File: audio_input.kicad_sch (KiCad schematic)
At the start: 7 parts

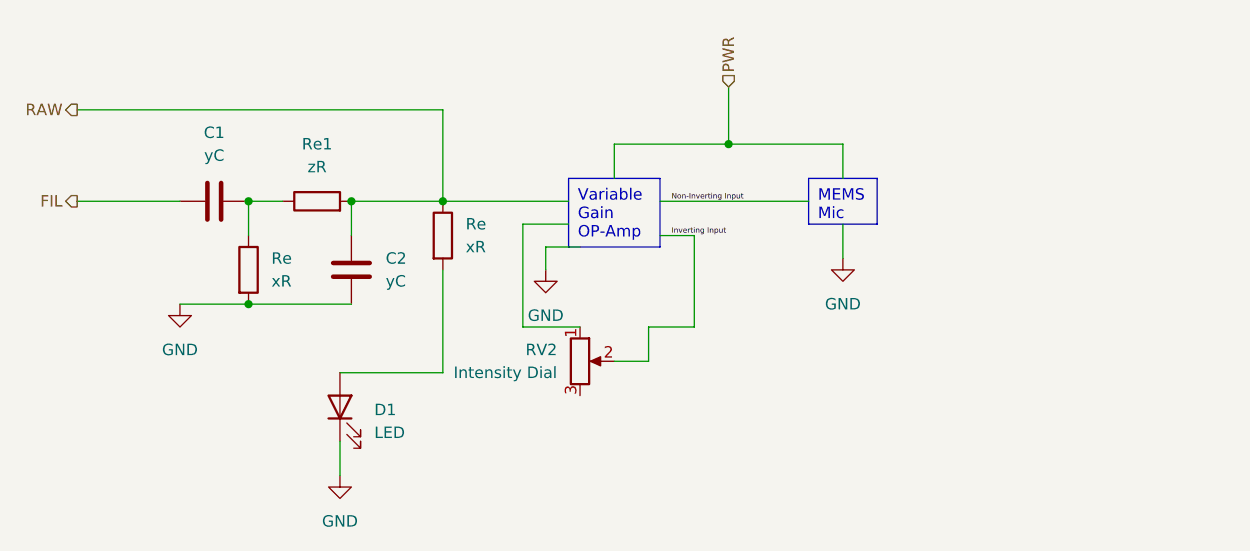
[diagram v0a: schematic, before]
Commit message: started work on pcb layout
started work on pcb layout
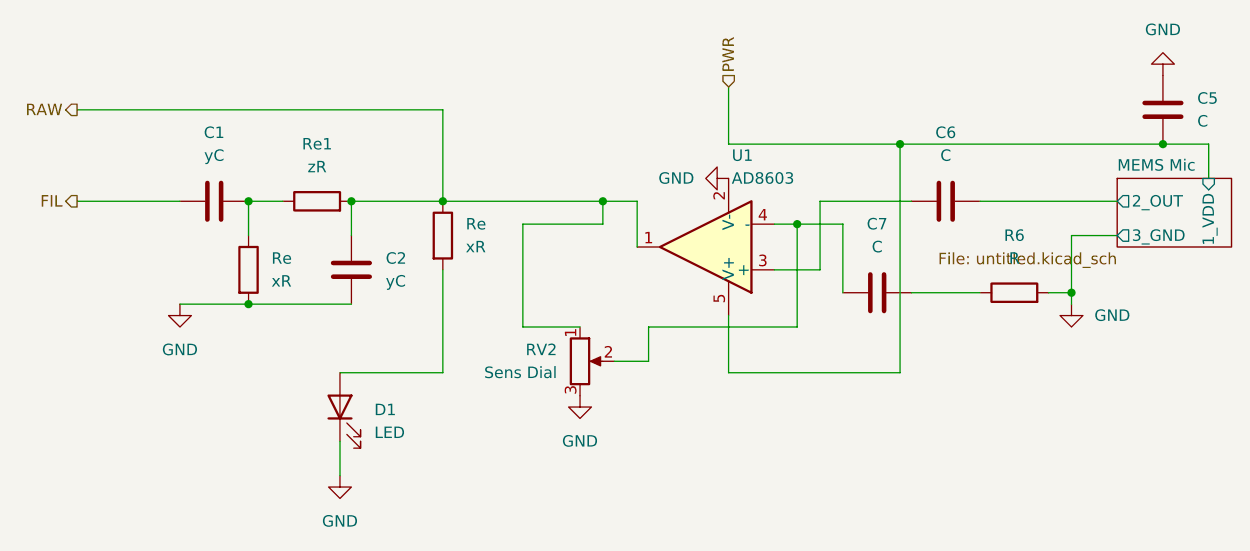
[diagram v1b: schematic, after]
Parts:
- added C5, C6, C7: C, Capacitor_SMD:C_0603_1608Metric_Pad1.08x0.95mm_HandSolder, symbol Device:C
- added R6: R, Resistor_SMD:R_0603_1608Metric_Pad0.98x0.95mm_HandSolder, symbol Device:R
- added U1: AD8603, Package_TO_SOT_SMD:TSOT-23-5, symbol Amplifier_Operational:AD8603
- RV2: value Intensity Dial -> Sens Dial
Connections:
- net GND: now also RV2.3, C5.1, R6.2, U1.2 (V-)
- net PWR: now also C5.2, U1.5 (V+)
- net RAW: now also RV2.1, U1.1
- net Inverting Input: no longer names the net of RV2.2
- net Inverting Input: now also C7.1, U1.4 (-)
- new net: C7.2, R6.1
- new net: C6.1, U1.3 (+)
- new net MEMS Mic/2_OUT: C6.2
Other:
- added sheet MEMS Mic (untitled.kicad_sch)
